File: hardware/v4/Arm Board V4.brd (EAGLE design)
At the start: 114.3 x 50.8 mm, 59 parts, among them IC3 L6206D, U1 SN74LS241DW, U2 XBEE-1B3, U3 LSM9DS0

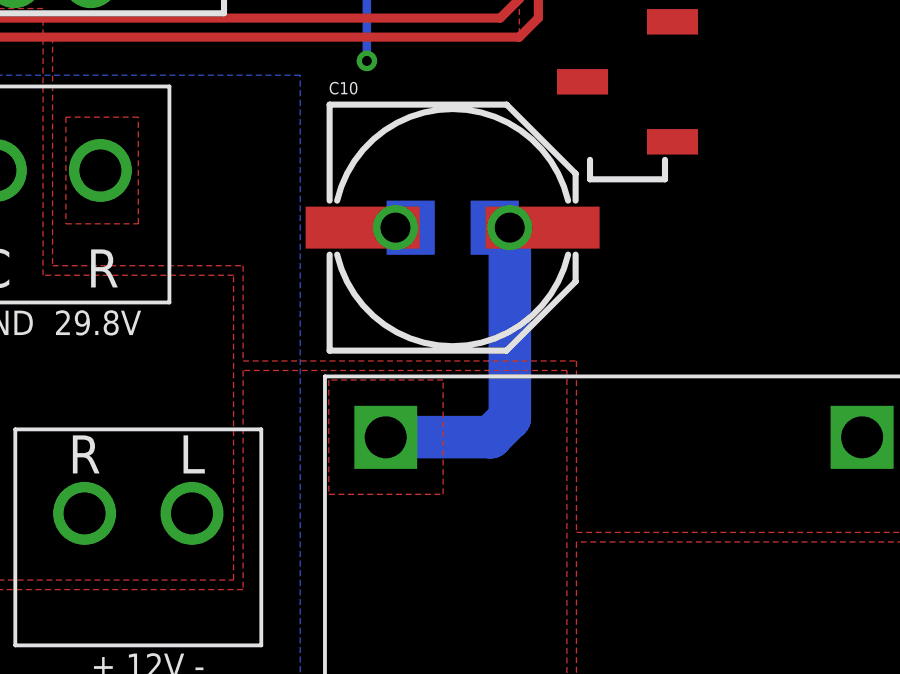
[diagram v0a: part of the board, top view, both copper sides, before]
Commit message: 32u4 Xbee Shield
32u4 Xbee Shield
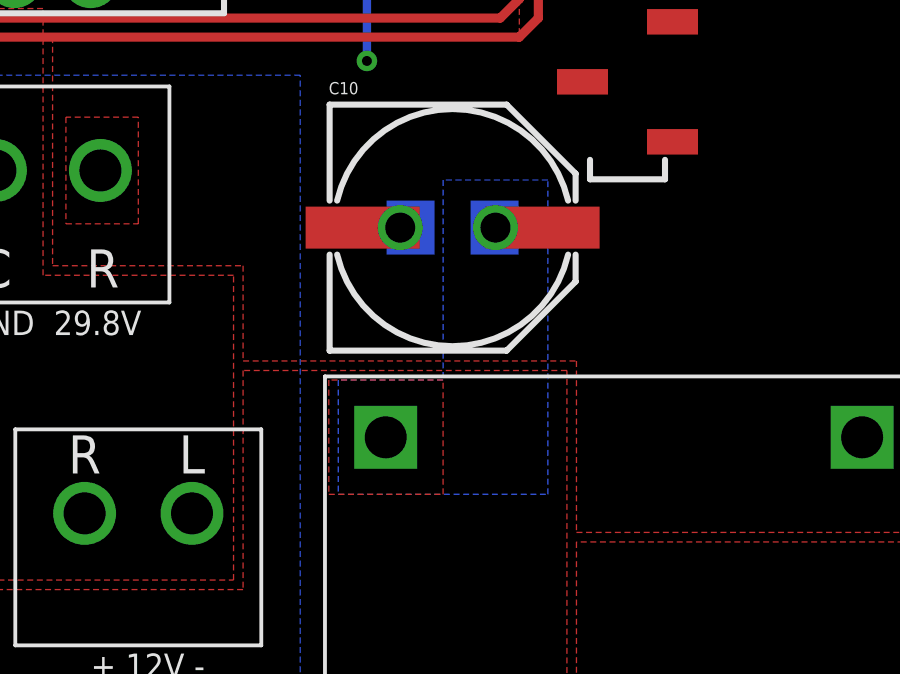
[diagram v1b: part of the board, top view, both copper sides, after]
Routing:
- net 14.8V: track 12.4 -> 1.57 mm
- added copper zone on layer 16, net 14.8V
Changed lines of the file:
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@@
 <setting verticaltext="up"/>
 </settings>
-<grid distance="0.05" unitdist="inch" unit="inch" style="lines" multiple="1" display="yes" altdistance="0.0125" altunitdist="inch" altunit="inch"/>
+<grid distance="0.05" unitdist="inch" unit="inch" style="lines" multiple="1" display="yes" altdistance="0.00625" altunitdist="inch" altunit="inch"/>
 <layers>
 <layer number="1" name="Top" color="4" fill="1" visible="yes" active="yes"/>
@@
 <contactref element="JP1" pad="4"/>
 <contactref element="C10" pad="-"/>
-<via x="70.485" y="27.94" extent="1-16" drill="1" shape="square"/>
+<via x="70.64375" y="27.94" extent="1-16" drill="1" shape="square"/>
 <contactref element="C1" pad="2"/>
 <contactref element="C3" pad="2"/>
@@
 <vertex x="114.3" y="11.1125"/>
 </polygon>
-<wire x1="70.485" y1="27.94" x2="69.39" y2="27.94" width="0.254" layer="1"/>
+<wire x1="70.64375" y1="27.94" x2="69.39" y2="27.94" width="0.254" layer="1"/>
 <contactref element="JP3" pad="4"/>
 <contactref element="JP2" pad="4"/>
@@
 <contactref element="JP12" pad="2"/>
 <contactref element="C10" pad="+"/>
-<via x="74.295" y="27.94" extent="1-16" drill="1" shape="square"/>
-<wire x1="74.295" y1="27.94" x2="74.295" y2="21.59" width="1.4224" layer="16"/>
-<wire x1="74.295" y1="21.59" x2="73.66" y2="20.955" width="1.4224" layer="16"/>
-<wire x1="73.66" y1="20.955" x2="70.165" y2="20.955" width="1.4224" layer="16"/>
-<wire x1="70.165" y1="20.955" x2="70.16" y2="20.95" width="1.4224" layer="16"/>
-<wire x1="75.39" y1="27.94" x2="74.295" y2="27.94" width="1.27" layer="1"/>
 <contactref element="C15" pad="1"/>
-<wire x1="73.79" y1="27.94" x2="74.295" y2="27.94" width="0.4064" layer="16"/>
+<polygon width="0.254" layer="16">
+<vertex x="68.58" y="22.86"/>
+<vertex x="68.58" y="19.05"/>
+<vertex x="75.565" y="19.05"/>
+<vertex x="75.565" y="29.5275"/>
+<vertex x="72.0725" y="29.5275"/>
+<vertex x="72.0725" y="22.86"/>
+</polygon>
+<via x="73.81875" y="27.94" extent="1-16" drill="1" shape="square"/>
+<wire x1="73.81875" y1="27.94" x2="75.39" y2="27.94" width="0.254" layer="1"/>
 </signal>
 <signal name="VIN">
